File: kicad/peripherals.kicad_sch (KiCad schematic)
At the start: 8 parts, among them P2 5k, U1 6526, U11 74ACT245, U2 W65C22SxP

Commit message: Uploaded firmware v2.0.2
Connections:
- net R~W renamed R~{W}
- net ~CIA renamed ~{CIA}
- net ~CIAEXT renamed ~{CIAEXT}
- net ~CIARES renamed ~{CIARES}
- net ~EXTFLAG renamed ~{EXTFLAG}
- net ~EXTPC renamed ~{EXTPC}
- net ~IRQ renamed ~{IRQ}
- net ~RES renamed ~{RES}
- net ~VIA renamed ~{VIA}
- net ~VIAIRQ renamed ~{VIAIRQ}

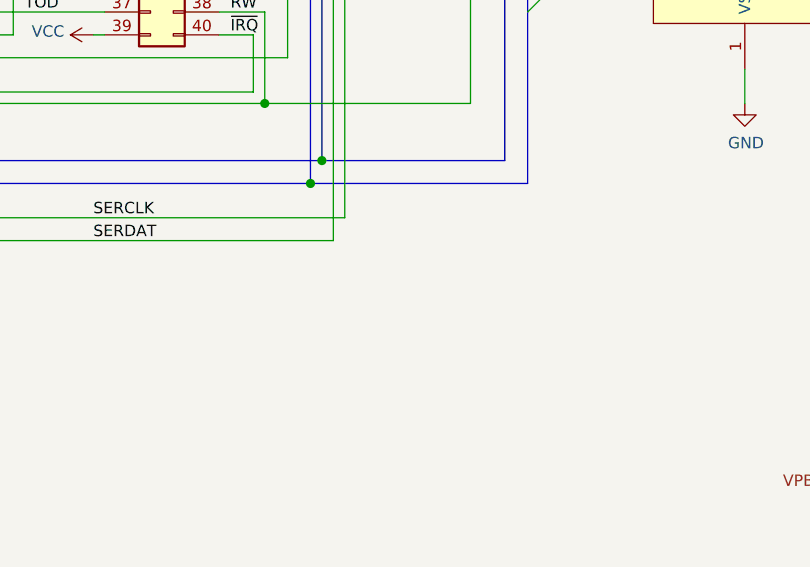
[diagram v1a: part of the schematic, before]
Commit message: PullUps con SERCLOCK and SERDAT
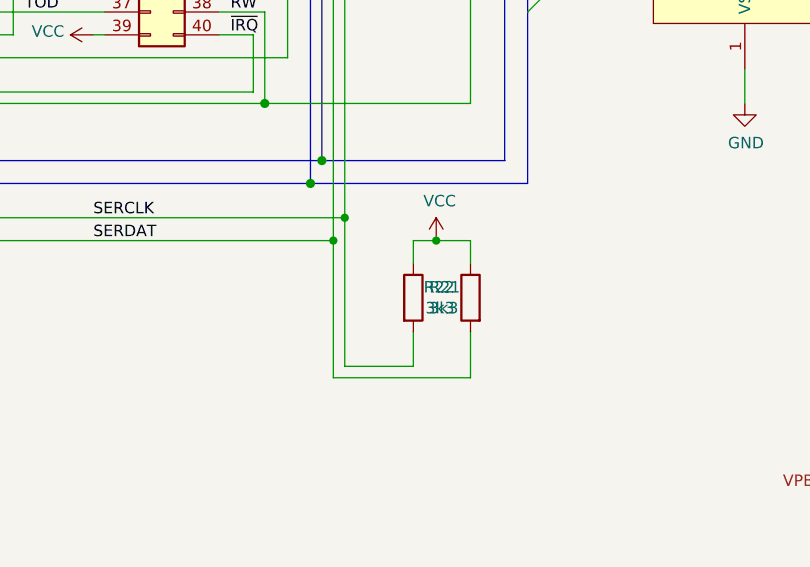
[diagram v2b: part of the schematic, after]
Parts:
- added R21, R22: 3k3, Resistor_SMD:R_0805_2012Metric_Pad1.20x1.40mm_HandSolder, symbol Device:R
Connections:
- net SERCLK: now also R21.2
- net SERDAT: now also R22.2
- net VCC: now also R21.1, R22.1
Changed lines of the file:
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@@
   (junction (at 46.99 121.92) (diameter 1.016) (color 0 0 0 0)
   )
+  (junction (at 175.26 137.16) (diameter 0) (color 0 0 0 0)
+  )
   (junction (at 156.21 121.92) (diameter 1.016) (color 0 0 0 0)
   )
@@
   (junction (at 38.1 57.15) (diameter 1.016) (color 0 0 0 0)
   )
+  (junction (at 165.1 134.62) (diameter 0) (color 0 0 0 0)
+  )
   (junction (at 156.21 33.02) (diameter 1.016) (color 0 0 0 0)
   )
@@
   )
   (junction (at 41.91 67.31) (diameter 1.016) (color 0 0 0 0)
+  )
+  (junction (at 163.83 137.16) (diameter 0) (color 0 0 0 0)
   )
   (no_connect (at 224.79 109.22))
@@
     (stroke (width 0) (type solid) (color 0 0 0 0))
   )
+  (wire (pts (xy 179.07 137.16) (xy 179.07 139.7))
+    (stroke (width 0) (type default) (color 0 0 0 0))
+  )
   (wire (pts (xy 128.27 93.98) (xy 138.43 93.98))
     (stroke (width 0) (type solid) (color 0 0 0 0))
@@
     (stroke (width 0) (type solid) (color 0 0 0 0))
   )
+  (wire (pts (xy 163.83 152.4) (xy 179.07 152.4))
+    (stroke (width 0) (type default) (color 0 0 0 0))
+  )
   (wire (pts (xy 88.9 59.69) (xy 119.38 59.69))
     (stroke (width 0) (type solid) (color 0 0 0 0))
@@
     (stroke (width 0) (type solid) (color 0 0 0 0))
   )
+  (wire (pts (xy 179.07 147.32) (xy 179.07 152.4))
+    (stroke (width 0) (type default) (color 0 0 0 0))
+  )
   (bus (pts (xy 125.73 104.14) (xy 125.73 106.68))
     (stroke (width 0) (type solid) (color 0 0 0 0))
@@
     (stroke (width 0) (type solid) (color 0 0 0 0))
   )
+  (wire (pts (xy 165.1 134.62) (xy 165.1 151.13))
+    (stroke (width 0) (type default) (color 0 0 0 0))
+  )
   (bus (pts (xy 185.42 111.76) (xy 185.42 130.81))
     (stroke (width 0) (type solid) (color 0 0 0 0))
@@
     (stroke (width 0) (type solid) (color 0 0 0 0))
   )
+  (wire (pts (xy 175.26 137.16) (xy 179.07 137.16))
+    (stroke (width 0) (type default) (color 0 0 0 0))
+  )
   (bus (pts (xy 243.84 91.44) (xy 243.84 93.98))
     (stroke (width 0) (type solid) (color 0 0 0 0))
@@
     (stroke (width 0) (type solid) (color 0 0 0 0))
   )
+  (wire (pts (xy 165.1 151.13) (xy 172.72 151.13))
+    (stroke (width 0) (type default) (color 0 0 0 0))
+  )
   (wire (pts (xy 265.43 76.2) (xy 265.43 77.47))
     (stroke (width 0) (type solid) (color 0 0 0 0))
@@
     (stroke (width 0) (type solid) (color 0 0 0 0))
   )
+  (wire (pts (xy 172.72 139.7) (xy 172.72 137.16))
+    (stroke (width 0) (type default) (color 0 0 0 0))
+  )
   (wire (pts (xy 46.99 121.92) (xy 156.21 121.92))
     (stroke (width 0) (type solid) (color 0 0 0 0))
@@
     (stroke (width 0) (type solid) (color 0 0 0 0))
   )
+  (wire (pts (xy 172.72 137.16) (xy 175.26 137.16))
+    (stroke (width 0) (type default) (color 0 0 0 0))
+  )
   (wire (pts (xy 194.31 104.14) (xy 187.96 104.14))
     (stroke (width 0) (type solid) (color 0 0 0 0))
@@
     (stroke (width 0) (type solid) (color 0 0 0 0))
   )
+  (wire (pts (xy 172.72 147.32) (xy 172.72 151.13))
+    (stroke (width 0) (type default) (color 0 0 0 0))
+  )
   (wire (pts (xy 224.79 60.96) (xy 236.22 60.96))
     (stroke (width 0) (type solid) (color 0 0 0 0))
@@
   (wire (pts (xy 124.46 111.76) (xy 124.46 35.56))
     (stroke (width 0) (type solid) (color 0 0 0 0))
+  )
+  (wire (pts (xy 163.83 137.16) (xy 163.83 152.4))
+    (stroke (width 0) (type default) (color 0 0 0 0))
   )
   (wire (pts (xy 39.37 62.23) (xy 35.56 62.23))
@@
     (pin "1")
   )
+  (symbol (lib_id "power:VCC") (at 175.26 137.16 0) (unit 1)
+    (in_bom yes) (on_board yes)
+    (property "Reference" "#PWR03" (id 0) (at 175.26 140.97 0)
+      (effects (font (size 1.27 1.27)) hide)
+    )
+    (property "Value" "VCC" (id 1) (at 175.641 132.7658 0))
+    (property "Footprint" "" (id 2) (at 175.26 137.16 0)
+      (effects (font (size 1.27 1.27)) hide)
+    )
+    (property "Datasheet" "" (id 3) (at 175.26 137.16 0)
+      (effects (font (size 1.27 1.27)) hide)
+    )
+    (pin "1")
+  )
   (symbol (lib_id "Device:R") (at 279.4 33.02 0) (unit 1)
     (in_bom yes) (on_board yes)
@@
       (effects (font (size 1.27 1.27)) hide)
     )
+    (pin "1")
+    (pin "2")
+  )
+  (symbol (lib_id "Device:R") (at 179.07 143.51 0) (mirror y) (unit 1)
+    (in_bom yes) (on_board yes)
+    (property "Reference" "R22" (id 0) (at 177.292 142.3416 0)
+      (effects (font (size 1.27 1.27)) (justify left))
+    )
+    (property "Value" "3k3" (id 1) (at 177.292 144.653 0)
+      (effects (font (size 1.27 1.27)) (justify left))
+    )
+    (property "Footprint" "Resistor_SMD:R_0805_2012Metric_Pad1.20x1.40mm_HandSolder" (id 2) (at 180.848 143.51 90)
+      (effects (font (size 1.27 1.27)) hide)
+    )
+    (property "Datasheet" "~" (id 3) (at 179.07 143.51 0)
+      (effects (font (size 1.27 1.27)) hide)
+    )
+    (pin "1")
+    (pin "2")
+  )
+  (symbol (lib_id "Device:R") (at 172.72 143.51 0) (unit 1)
+    (in_bom yes) (on_board yes)
+    (property "Reference" "R21" (id 0) (at 174.498 142.3416 0)
+      (effects (font (size 1.27 1.27)) (justify left))
+    )
+    (property "Value" "3k3" (id 1) (at 174.498 144.653 0)
+      (effects (font (size 1.27 1.27)) (justify left))
+    )
+    (property "Footprint" "Resistor_SMD:R_0805_2012Metric_Pad1.20x1.40mm_HandSolder" (id 2) (at 170.942 143.51 90)
+      (effects (font (size 1.27 1.27)) hide)
+    )
+    (property "Datasheet" "~" (id 3) (at 172.72 143.51 0)
+      (effects (font (size 1.27 1.27)) hide)
+    )
